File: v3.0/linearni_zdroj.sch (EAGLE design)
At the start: 38 parts, among them IC1 LM358N, IC2 LM358N, Q1 IRFZ34NAV, Q2 TIP120

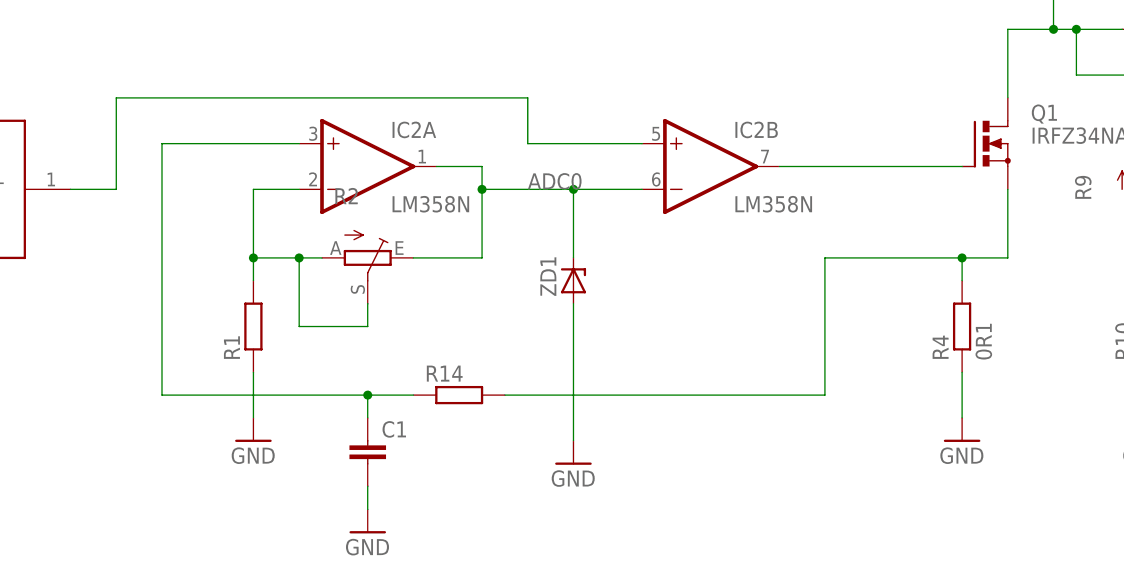
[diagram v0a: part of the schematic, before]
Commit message: zase sem se jednou ve škole něco naučil
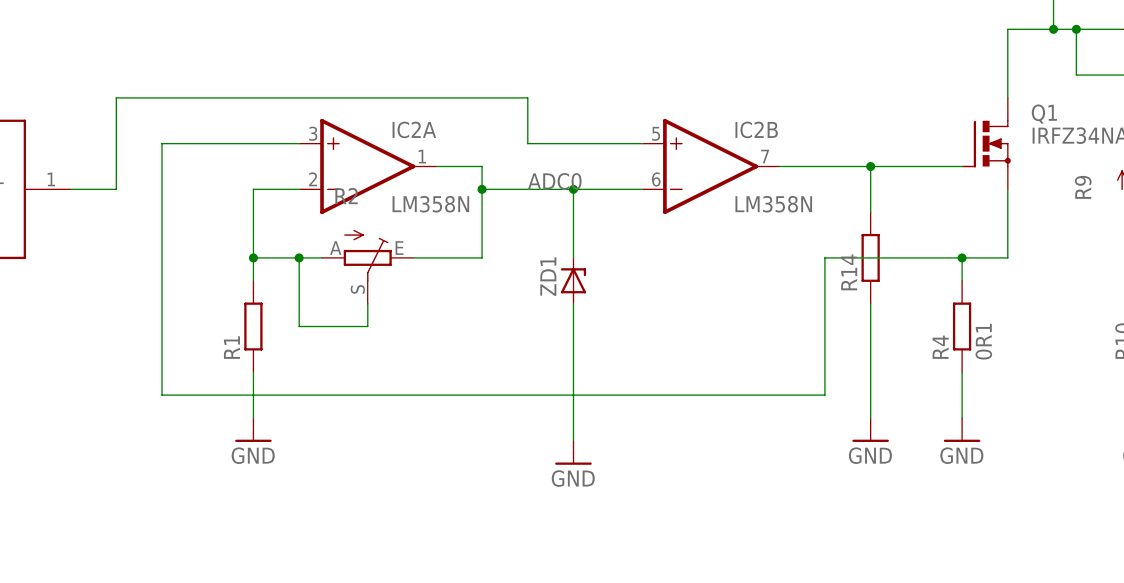
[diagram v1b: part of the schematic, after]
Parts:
- removed C1: (no value), rcl:C-EUC0805
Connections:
- removed net N$1: Q1.S, R14.2, R4.2
- net GND: now also R14.1; no longer C1.2
- net N$2: now also R14.2
- net N$20: now also Q1.S, R4.2; no longer C1.1, R14.1
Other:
- moved on the sheet: R14
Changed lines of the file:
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@@
 <part name="+3V6" library="supply1" library_urn="urn:adsk.eagle:library:371" deviceset="+3V3" device=""/>
 <part name="+3V7" library="supply1" library_urn="urn:adsk.eagle:library:371" deviceset="+3V3" device=""/>
-<part name="R14" library="rcl" library_urn="urn:adsk.eagle:library:334" deviceset="R-EU_" device="R0805" package3d_urn="urn:adsk.eagle:package:23553/2"/>
-<part name="C1" library="rcl" library_urn="urn:adsk.eagle:library:334" deviceset="C-EU" device="C0805" package3d_urn="urn:adsk.eagle:package:23617/2"/>
-<part name="GND8" library="supply1" library_urn="urn:adsk.eagle:library:371" deviceset="GND" device=""/>
 <part name="Q1" library="devices" deviceset="IRFZ34N" device="AV" override_package3d_urn="urn:adsk.eagle:package:33936961/2" override_package_urn="urn:adsk.eagle:footprint:33936962/1"/>
 <part name="P+5" library="supply1" library_urn="urn:adsk.eagle:library:371" deviceset="+24V" device=""/>
@@
 <part name="C2" library="rcl" library_urn="urn:adsk.eagle:library:334" deviceset="C-EU" device="C0805" package3d_urn="urn:adsk.eagle:package:23617/2" value="10n"/>
 <part name="+3V8" library="supply1" library_urn="urn:adsk.eagle:library:371" deviceset="+3V3" device=""/>
+<part name="GND8" library="supply1" library_urn="urn:adsk.eagle:library:371" deviceset="GND" device=""/>
+<part name="R14" library="rcl" library_urn="urn:adsk.eagle:library:334" deviceset="R-EU_" device="R0805" package3d_urn="urn:adsk.eagle:package:23553/2"/>
 </parts>
 <sheets>
@@
 <attribute name="VALUE" x="269.24" y="154.94" size="1.778" layer="96" rot="R180"/>
 </instance>
-<instance part="R14" gate="G$1" x="50.8" y="27.94" smashed="yes">
-<attribute name="NAME" x="46.99" y="29.4386" size="1.778" layer="95"/>
-<attribute name="VALUE" x="46.99" y="24.638" size="1.778" layer="96"/>
-</instance>
-<instance part="C1" gate="G$1" x="40.64" y="22.86" smashed="yes">
-<attribute name="NAME" x="42.164" y="23.241" size="1.778" layer="95"/>
-<attribute name="VALUE" x="42.164" y="18.161" size="1.778" layer="96"/>
-</instance>
-<instance part="GND8" gate="1" x="40.64" y="12.7" smashed="yes">
-<attribute name="VALUE" x="38.1" y="10.16" size="1.778" layer="96"/>
-</instance>
 <instance part="Q1" gate="G$1" x="109.22" y="55.88" smashed="yes">
 <attribute name="NAME" x="114.3" y="58.42" size="1.778" layer="95"/>
@@
 <instance part="+3V8" gate="G$1" x="287.02" y="149.86" smashed="yes">
 <attribute name="VALUE" x="289.56" y="152.4" size="1.778" layer="96" rot="R180"/>
+</instance>
+<instance part="GND8" gate="1" x="96.52" y="22.86" smashed="yes">
+<attribute name="VALUE" x="93.98" y="20.32" size="1.778" layer="96"/>
+</instance>
+<instance part="R14" gate="G$1" x="96.52" y="43.18" smashed="yes" rot="R90">
+<attribute name="NAME" x="95.0214" y="39.37" size="1.778" layer="95" rot="R90"/>
+<attribute name="VALUE" x="99.822" y="39.37" size="1.778" layer="96" rot="R90"/>
 </instance>
 </instances>
@@
 </busses>
 <nets>
-<net name="N$1" class="0">
-<segment>
-<wire x1="111.76" y1="43.18" x2="106.68" y2="43.18" width="0.1524" layer="91"/>
-<wire x1="106.68" y1="43.18" x2="91.44" y2="43.18" width="0.1524" layer="91"/>
-<wire x1="91.44" y1="43.18" x2="91.44" y2="27.94" width="0.1524" layer="91"/>
-<pinref part="R4" gate="G$1" pin="2"/>
-<wire x1="106.68" y1="40.64" x2="106.68" y2="43.18" width="0.1524" layer="91"/>
-<junction x="106.68" y="43.18"/>
-<wire x1="111.76" y1="50.8" x2="111.76" y2="43.18" width="0.1524" layer="91"/>
-<wire x1="91.44" y1="27.94" x2="55.88" y2="27.94" width="0.1524" layer="91"/>
-<pinref part="R14" gate="G$1" pin="2"/>
-<pinref part="Q1" gate="G$1" pin="S"/>
-</segment>
-</net>
 <net name="N$3" class="0">
 <segment>
@@
 <segment>
 <pinref part="GND8" gate="1" pin="GND"/>
-<pinref part="C1" gate="G$1" pin="2"/>
-<wire x1="40.64" y1="15.24" x2="40.64" y2="17.78" width="0.1524" layer="91"/>
+<wire x1="96.52" y1="25.4" x2="96.52" y2="38.1" width="0.1524" layer="91"/>
+<pinref part="R14" gate="G$1" pin="1"/>
 </segment>
 </net>
@@
 <wire x1="17.78" y1="55.88" x2="33.02" y2="55.88" width="0.1524" layer="91"/>
 <wire x1="17.78" y1="27.94" x2="17.78" y2="55.88" width="0.1524" layer="91"/>
-<wire x1="45.72" y1="27.94" x2="40.64" y2="27.94" width="0.1524" layer="91"/>
-<pinref part="R14" gate="G$1" pin="1"/>
-<pinref part="C1" gate="G$1" pin="1"/>
-<wire x1="40.64" y1="27.94" x2="17.78" y2="27.94" width="0.1524" layer="91"/>
-<wire x1="40.64" y1="25.4" x2="40.64" y2="27.94" width="0.1524" layer="91"/>
-<junction x="40.64" y="27.94"/>
+<wire x1="91.44" y1="27.94" x2="17.78" y2="27.94" width="0.1524" layer="91"/>
+<wire x1="111.76" y1="43.18" x2="106.68" y2="43.18" width="0.1524" layer="91"/>
+<wire x1="106.68" y1="43.18" x2="91.44" y2="43.18" width="0.1524" layer="91"/>
+<wire x1="91.44" y1="43.18" x2="91.44" y2="27.94" width="0.1524" layer="91"/>
+<pinref part="R4" gate="G$1" pin="2"/>
+<wire x1="106.68" y1="40.64" x2="106.68" y2="43.18" width="0.1524" layer="91"/>
+<junction x="106.68" y="43.18"/>
+<wire x1="111.76" y1="50.8" x2="111.76" y2="43.18" width="0.1524" layer="91"/>
+<pinref part="Q1" gate="G$1" pin="S"/>
 </segment>
 </net>
@@
 <pinref part="IC2" gate="B" pin="OUT"/>
 <pinref part="Q1" gate="G$1" pin="G"/>
-<wire x1="86.36" y1="53.34" x2="106.68" y2="53.34" width="0.1524" layer="91"/>
-</segment>
-</net>
+<wire x1="86.36" y1="53.34" x2="96.52" y2="53.34" width="0.1524" layer="91"/>
+<pinref part="R14" gate="G$1" pin="2"/>
+<wire x1="96.52" y1="53.34" x2="106.68" y2="53.34" width="0.1524" layer="91"/>
+<wire x1="96.52" y1="48.26" x2="96.52" y2="53.34" width="0.1524" layer="91"/>
+<junction x="96.52" y="53.34"/>
+</segment>
+</net>
